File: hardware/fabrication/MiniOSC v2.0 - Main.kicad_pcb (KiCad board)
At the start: 2 copper layers, 65 x 128.5 mm, 82 parts, among them J1 SYNC_IN, J10 FM_IN, J11 PWM_CV, J12 TRI_OUT, J13 SAW_OUT, J14 PULSE_OUT, J2 Conn_01x10_Pin, J9 VOCT_IN, Q3 BC848, Q4 BC858, SW1 SW_DPDT_x2, U1 40106, U2 TL074, U3 TL074

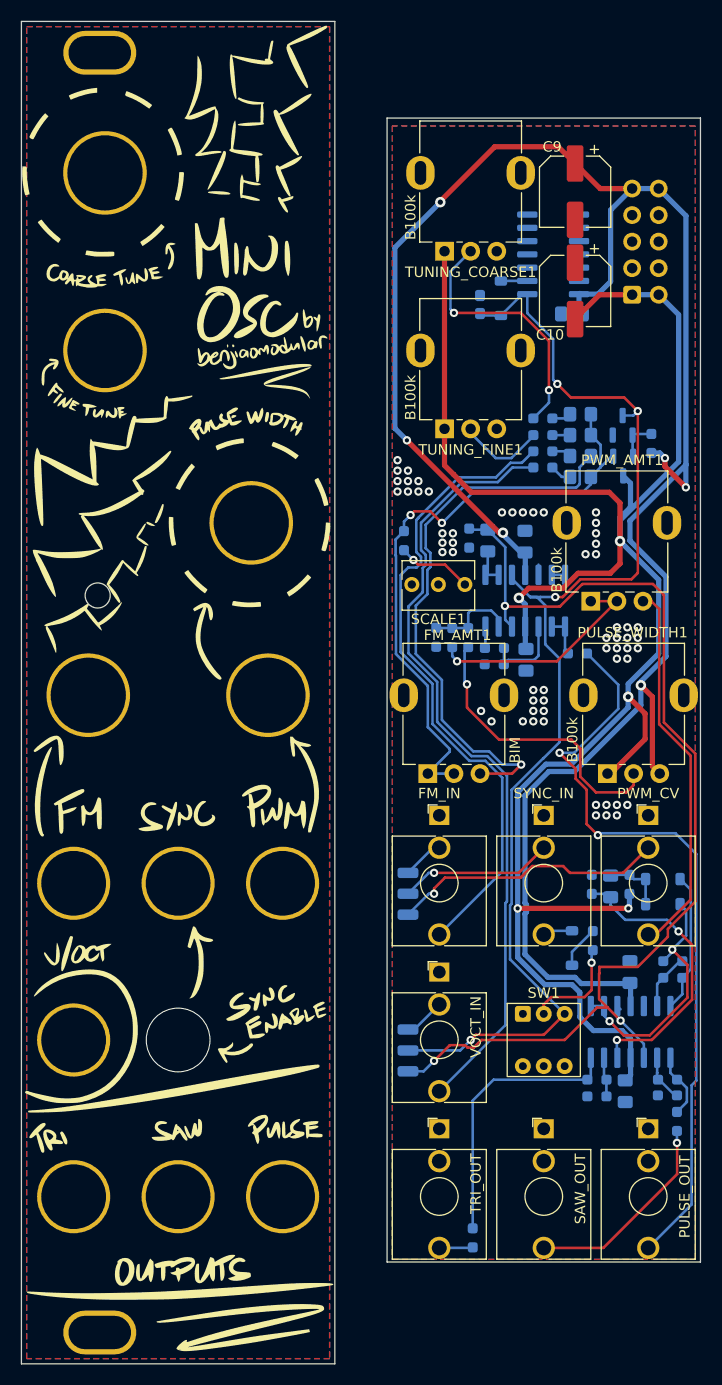
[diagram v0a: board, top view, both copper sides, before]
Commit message: v2.0 PCB
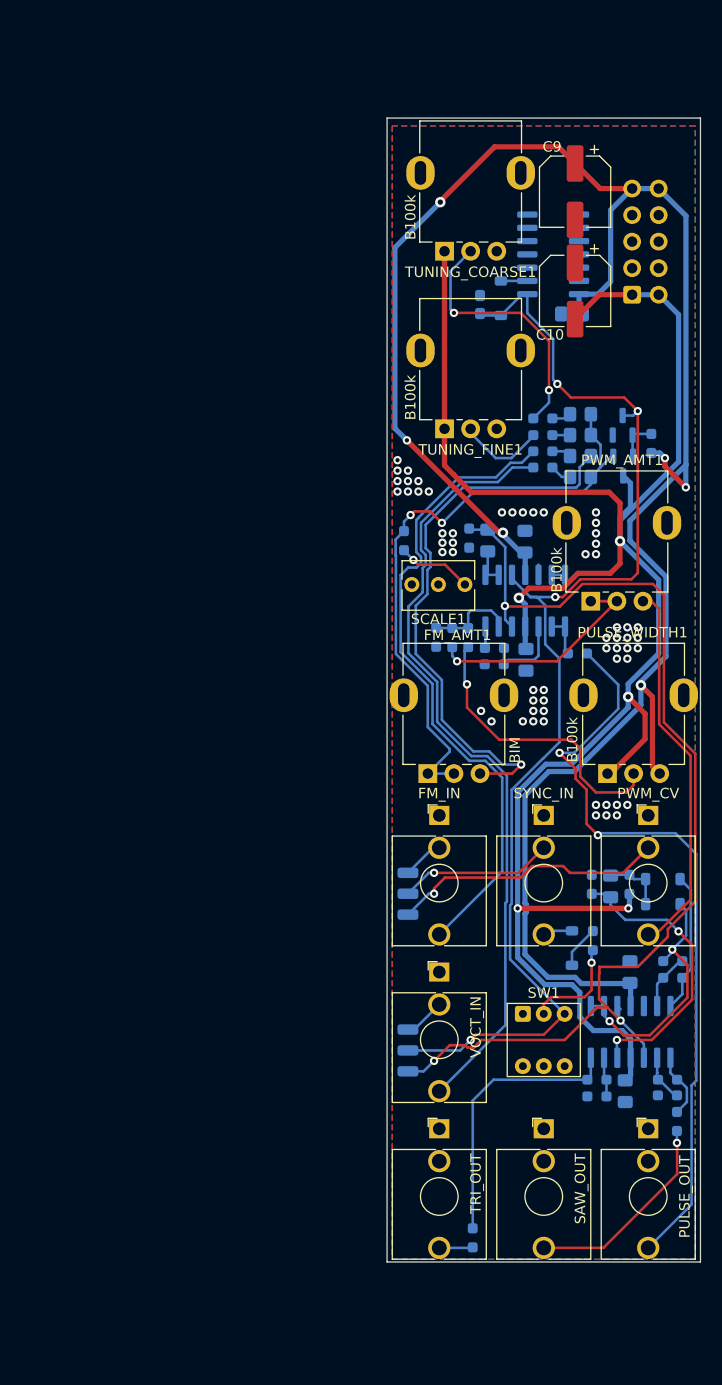
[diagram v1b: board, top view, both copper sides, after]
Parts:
- removed G***: LOGO, LOGO
- removed REF** (x5): PanelHole_Potentiometer_RV09, benjiaomodular:PanelHole_Potentiometer_RV09
- removed REF** (x7): PanelHole_AudioJack_3.5mm, benjiaomodular:PanelHole_AudioJack_3.5mm
- removed REF**: Panel_6HP, benjiaomodular:Panel_6HP
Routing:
- net (no net): vias 1 -> 0
- removed copper zone on B.Cu, net (none)
- removed copper zone on F.Cu, net (none)
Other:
- board size 65 x 128.5 mm -> 30 x 109.5 mm
